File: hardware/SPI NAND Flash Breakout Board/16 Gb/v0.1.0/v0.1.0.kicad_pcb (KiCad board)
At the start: 2 copper layers, 40 x 30 mm, 18 parts, among them J1 Conn_01x09_Pin, U1 AS5F18G04SND-10LIN, U2 AS5F18G04SND-10LIN, U3 TXB0108PW, U4 AP2127K-1.8

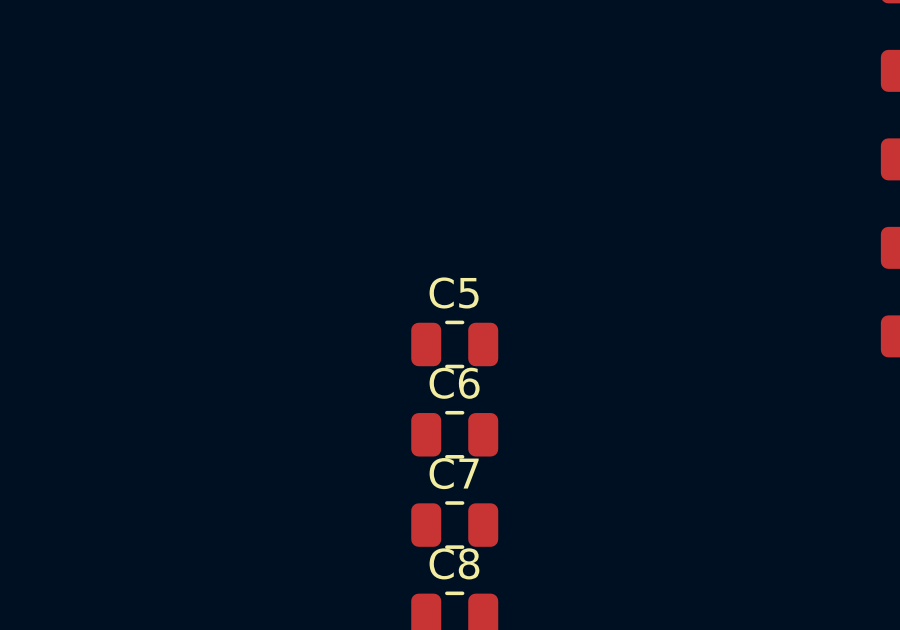
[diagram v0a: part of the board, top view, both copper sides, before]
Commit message: org
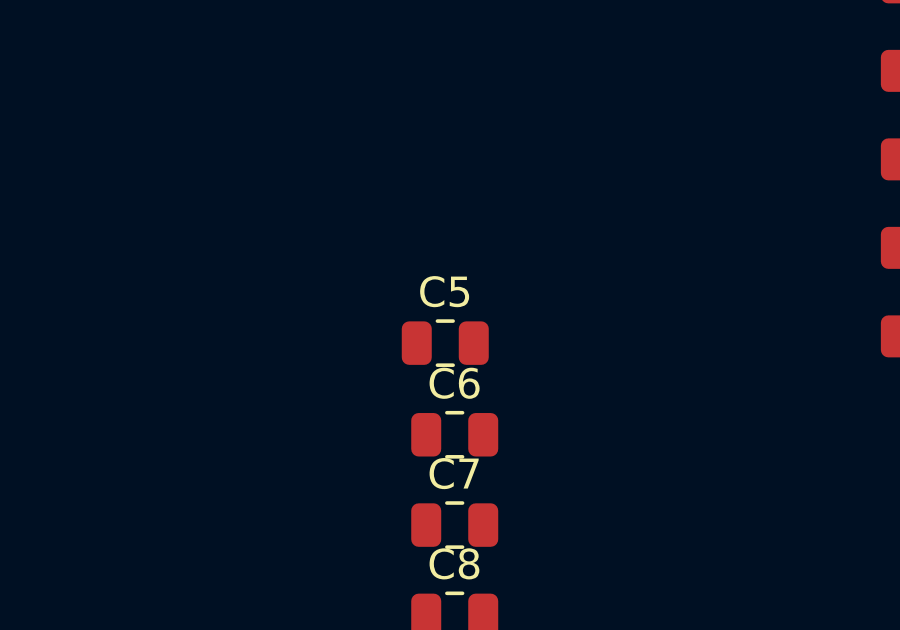
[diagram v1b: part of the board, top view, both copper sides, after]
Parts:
- moved C5 0.32 mm to (139.0, 88.0)
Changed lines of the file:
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@@
 	(footprint "Capacitor_SMD:C_0805_2012Metric"
 		(layer "F.Cu")
-		(at 139.315 88.045)
+		(at 139 88)
 		(descr "Capacitor SMD 0805 (2012 Metric), square (rectangular) end terminal, IPC-7351 nominal, (Body size source: IPC-SM-782 page 76, https://www.pcb-3d.com/wordpress/wp-content/uploads/ipc-sm-782a_amendment_1_and_2.pdf, https://docs.google.com/spreadsheets/d/1BsfQQcO9C6DZCsRaXUlFlo91Tg2WpOkGARC1WS5S8t0/edit?usp=sharing)")
 		(tags "capacitor")
@@
 	)
 	(segment
+		(start 115.968077 124.05)
+		(end 116 124.081923)
+		(width 0.35)
+		(layer "F.Cu")
+		(net "Net-(U1-VCC)")
+	)
+	(segment
+		(start 117.05 119.5)
+		(end 117.05 117.325)
+		(width 0.35)
+		(layer "F.Cu")
+		(net "Net-(U1-VCC)")
+	)
+	(segment
+		(start 116 124.081923)
+		(end 116 117.275)
+		(width 0.35)
+		(layer "F.Cu")
+		(net "Net-(U1-VCC)")
+	)
+	(segment
+		(start 117.05 117.325)
+		(end 117 117.275)
+		(width 0.35)
+		(layer "F.Cu")
+		(net "Net-(U1-VCC)")
+	)
+	(segment
+		(start 117 117.275)
+		(end 118.8625 117.275)
+		(width 0.35)
+		(layer "F.Cu")
+		(net "Net-(U1-VCC)")
+	)
+	(segment
+		(start 113.1375 124.05)
+		(end 115.968077 124.05)
+		(width 0.35)
+		(layer "F.Cu")
+		(net "Net-(U1-VCC)")
+	)
+	(segment
+		(start 116 117.275)
+		(end 117 117.275)
+		(width 0.35)
+		(layer "F.Cu")
+		(net "Net-(U1-VCC)")
+	)
+	(segment
 		(start 107.05 125.7)
 		(end 107.05 128)
@@
 		(net "Net-(J1-Pin_9)")
 	)
-	(segment
-		(start 115.968077 124.05)
-		(end 116 124.081923)
-		(width 0.35)
-		(layer "F.Cu")
-		(net "Net-(U1-VCC)")
-	)
-	(segment
-		(start 117.05 119.5)
-		(end 117.05 117.325)
-		(width 0.35)
-		(layer "F.Cu")
-		(net "Net-(U1-VCC)")
-	)
-	(segment
-		(start 116 124.081923)
-		(end 116 117.275)
-		(width 0.35)
-		(layer "F.Cu")
-		(net "Net-(U1-VCC)")
-	)
-	(segment
-		(start 117.05 117.325)
-		(end 117 117.275)
-		(width 0.35)
-		(layer "F.Cu")
-		(net "Net-(U1-VCC)")
-	)
-	(segment
-		(start 117 117.275)
-		(end 118.8625 117.275)
-		(width 0.35)
-		(layer "F.Cu")
-		(net "Net-(U1-VCC)")
-	)
-	(segment
-		(start 113.1375 124.05)
-		(end 115.968077 124.05)
-		(width 0.35)
-		(layer "F.Cu")
-		(net "Net-(U1-VCC)")
-	)
-	(segment
-		(start 116 117.275)
-		(end 117 117.275)
-		(width 0.35)
-		(layer "F.Cu")
-		(net "Net-(U1-VCC)")
-	)
 	(zone
